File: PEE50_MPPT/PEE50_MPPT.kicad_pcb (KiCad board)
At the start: 2 copper layers, 125 x 125 mm, 172 parts, among them J1 Vout, J2 Conn_01x02_Female, J3 Conn_01x03_Female, J4 Conn_01x03_Female, J5 PV_IN1, J6 PV_IN1, J7 PV_IN1, J8 PV_IN1, Q1 BC547, Q2 BC547, Q3 BC547, Q4 BC547, U1 LM3480-3.3, U10 NTA4151PT1G, U11 CSD18514Q5A, U12 CSD18543Q3A, U13 TPS552882QRPMRQ1, U14 MAX44284FAUT+T, U15 MAX44284FAUT+T, U16 NTA4151PT1G, U17 CSD18514Q5A, U18 CSD18543Q3A, U19 TPS552882QRPMRQ1, U2 MSP430FR2353TDBT, U20 MAX44284FAUT+T, U21 MAX44284FAUT+T, U22 NTA4151PT1G, U23 CSD18514Q5A, U24 CSD18543Q3A, U25 TPS552882QRPMRQ1, U26 MAX44284FAUT+T, U27 MAX44284FAUT+T, U3 ADG706BRUZ, U4 NTA4151PT1G, U5 CSD18514Q5A, U6 CSD18543Q3A, U7 TPS552882QRPMRQ1, U8 MAX44284FAUT+T, U9 MAX44284FAUT+T

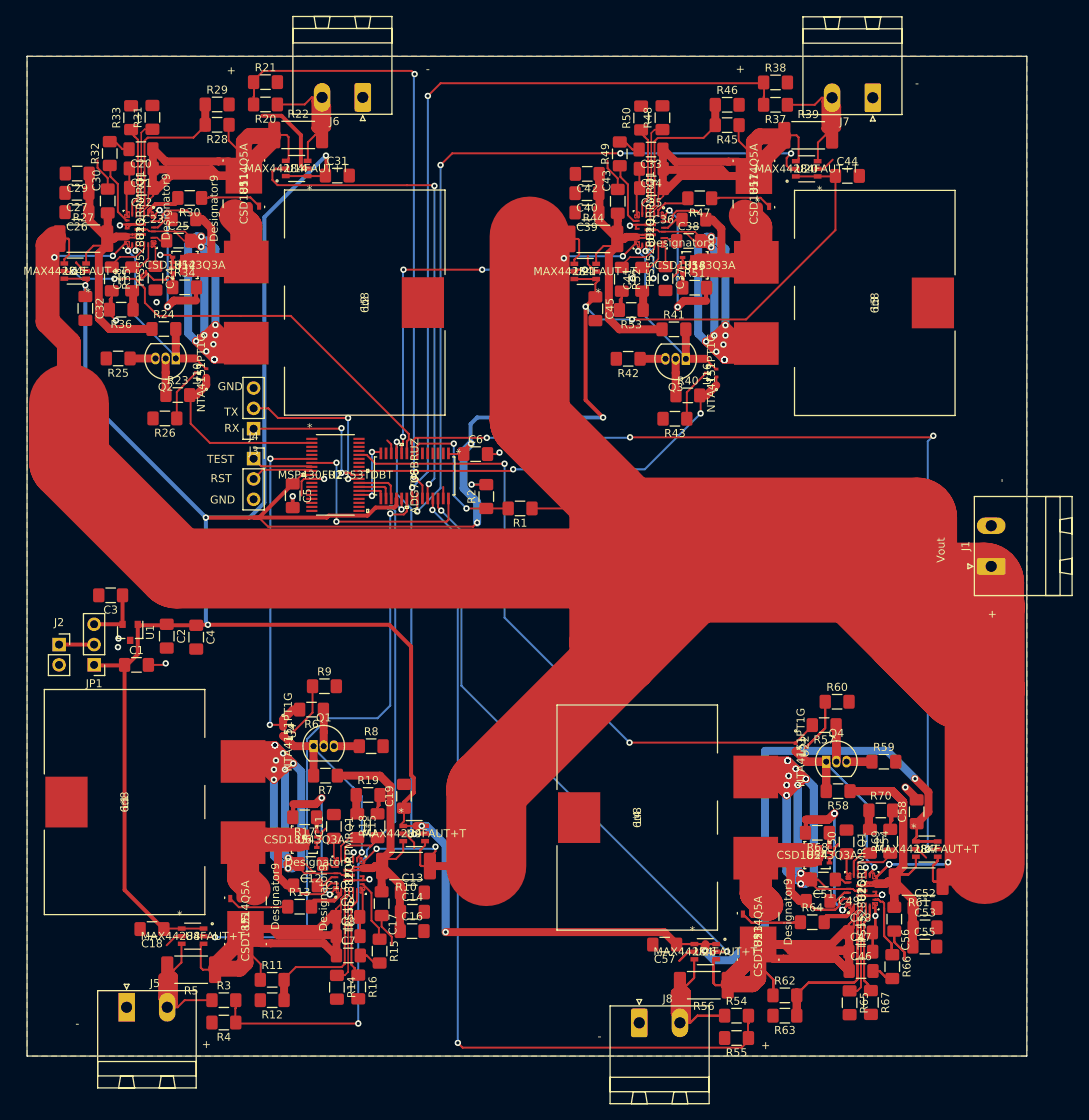
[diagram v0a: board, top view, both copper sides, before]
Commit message: heel wat silkscreen gefixt
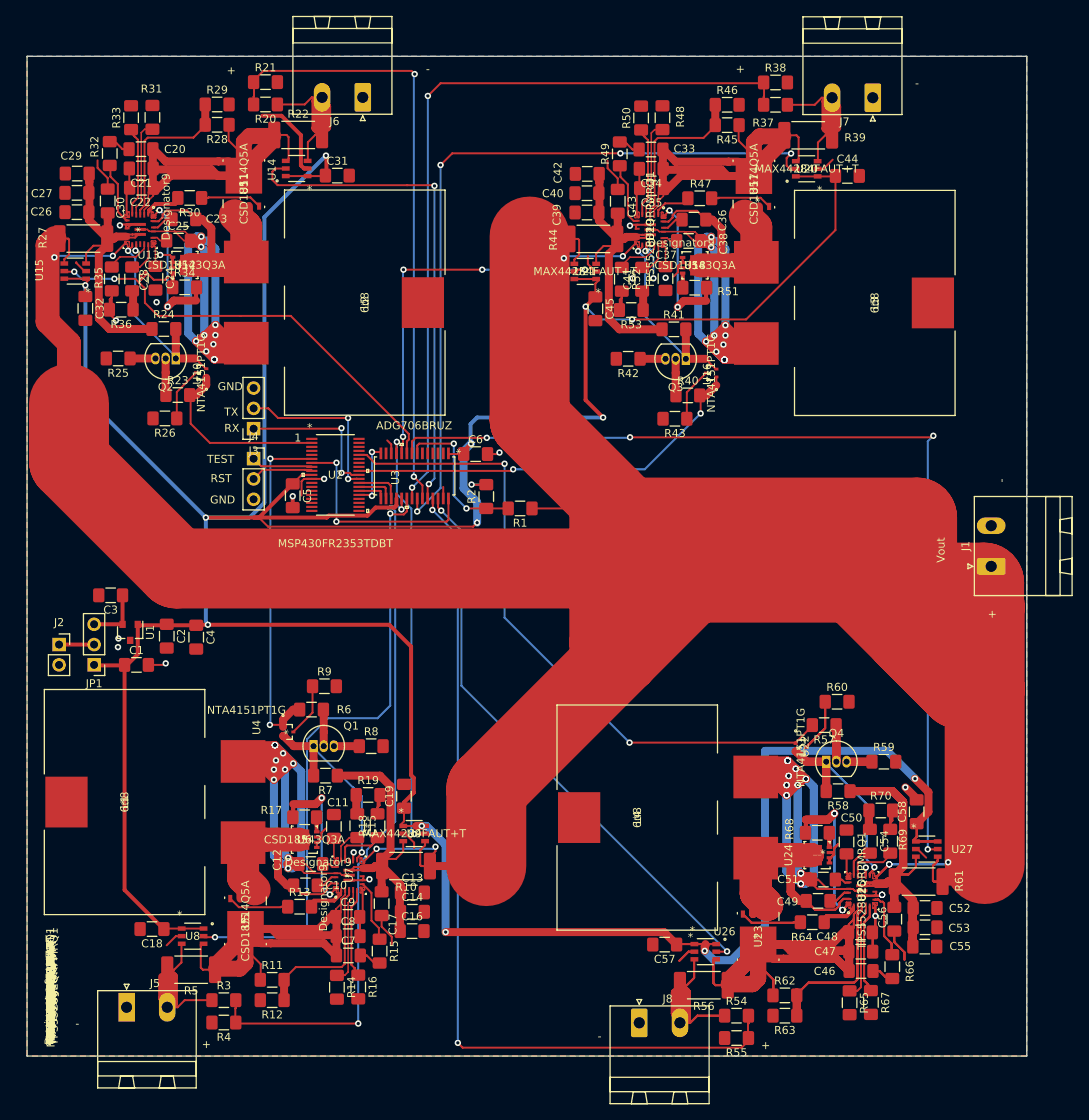
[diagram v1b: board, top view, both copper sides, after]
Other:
- board text added: "1"
